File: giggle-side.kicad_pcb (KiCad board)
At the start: 2 copper layers, 97.5 x 97 mm, 41 parts, among them J2 CONN_05X2SHD

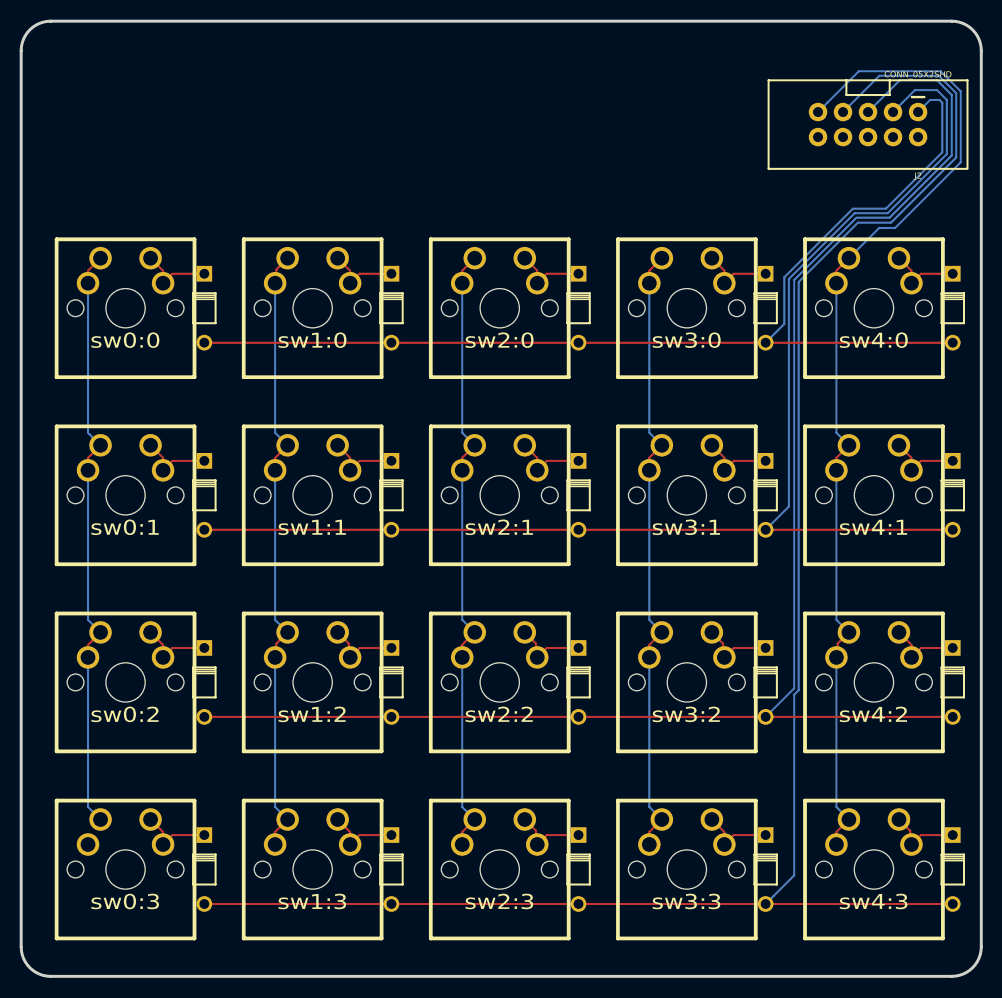
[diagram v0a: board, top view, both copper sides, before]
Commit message: placed the switches and stuff in the main, i guess.
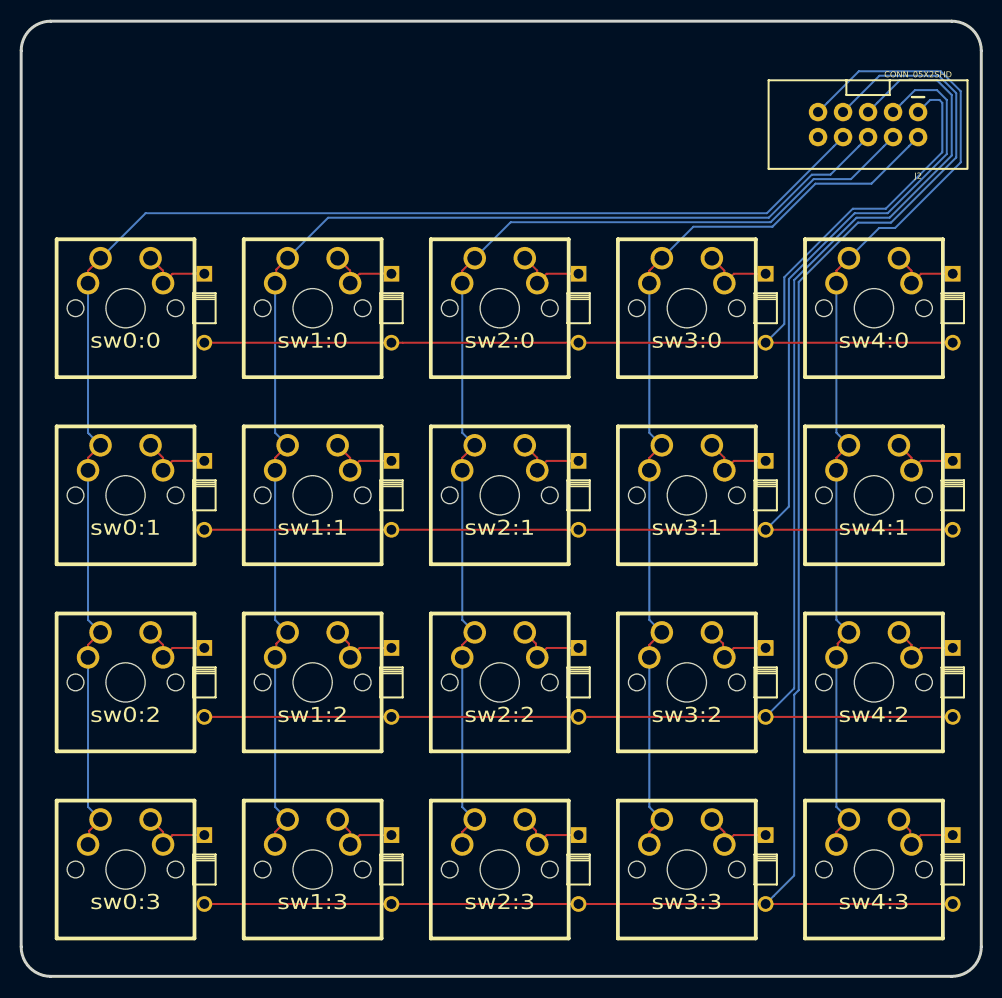
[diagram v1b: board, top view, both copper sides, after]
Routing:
- net N-col-0: track 60.2 -> 143.7 mm
- net N-col-1: track 63.2 -> 127.3 mm
- net N-col-2: track 63.2 -> 110.8 mm
- net N-col-3: track 63.2 -> 94.3 mm
- net N-col-8: track 0.00 -> 7.65 mm
- net N-col-7: track 0.00 -> 7.65 mm
- net N-col-6: track 0.00 -> 7.65 mm
- net N-col-5: track 0.00 -> 7.65 mm
- net N-col-11: track 0.00 -> 7.65 mm
- net N-diode-19: track 7.65 -> 0.00 mm
- net N-diode-14: track 7.65 -> 0.00 mm
- net N-diode-11: track 7.65 -> 0.00 mm
- net N-col-9: track 0.00 -> 7.65 mm
- net N-col-12: track 0.00 -> 7.65 mm
- net N-col-10: track 0.00 -> 7.65 mm
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
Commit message: finished main side.
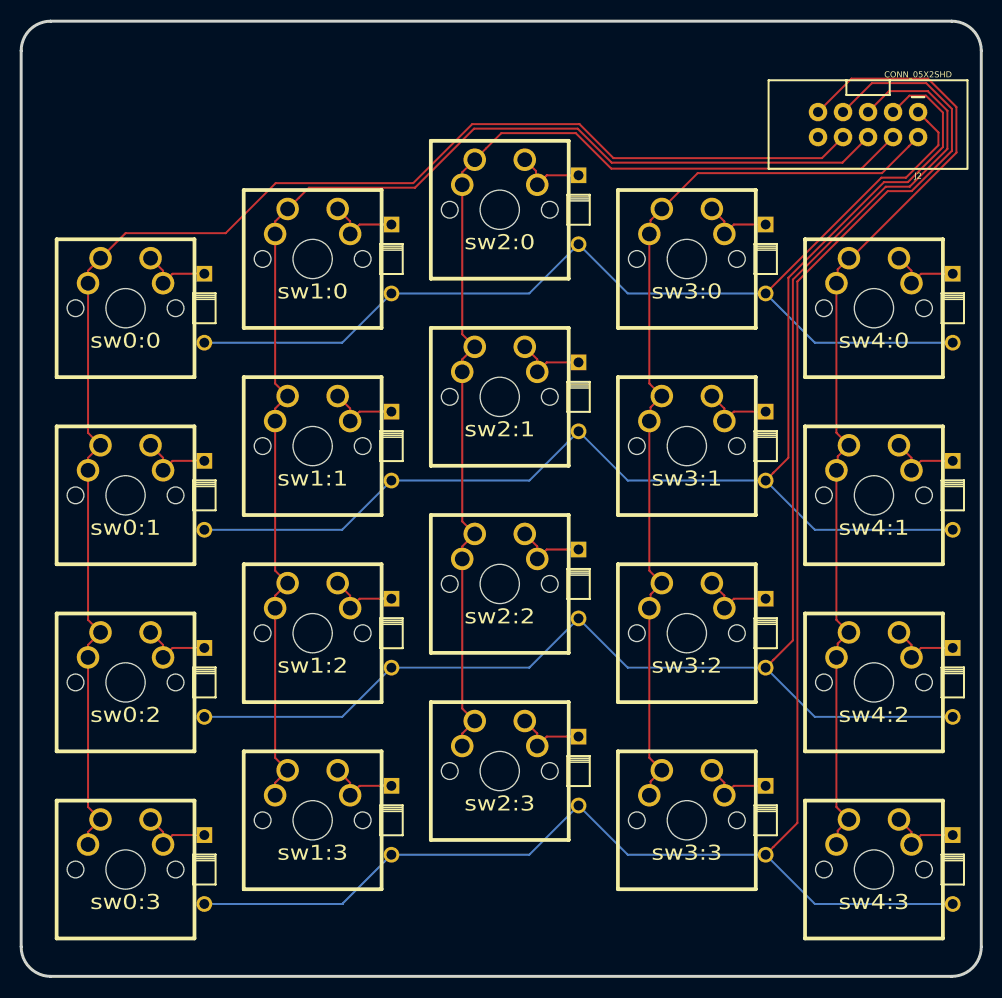
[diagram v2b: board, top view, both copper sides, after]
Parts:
- moved d2:0 10.0 mm to (84.1, 47.1)
- moved d2:1 10.0 mm to (84.1, 66.2)
- moved d2:2 10.0 mm to (84.1, 85.2)
- moved d2:3 10.0 mm to (84.1, 104.2)
- moved sw2:0 10.0 mm to (76.1, 47.1)
- moved sw2:1 10.0 mm to (76.1, 66.2)
- moved sw2:2 10.0 mm to (76.1, 85.2)
- moved sw2:3 10.0 mm to (76.1, 104.2)
- moved d1:0 5.00 mm to (65.1, 52.1)
- moved d1:1 5.00 mm to (65.1, 71.2)
- moved d1:2 5.00 mm to (65.1, 90.2)
- moved d1:3 5.00 mm to (65.1, 109.2)
- moved d3:0 5.00 mm to (103.1, 52.1)
- moved d3:1 5.00 mm to (103.1, 71.2)
- moved d3:2 5.00 mm to (103.1, 90.2)
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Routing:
- net N-col-4: track 102.9 -> 99.9 mm
- net N-col-0: track 143.7 -> 146.6 mm
- net N-col-3: track 94.3 -> 92.3 mm
- net N-col-2: track 110.8 -> 109.6 mm
- net N-row-1: track 136.0 -> 137.0 mm
- net N-row-3: track 182.1 -> 183.0 mm
- net N-col-1: track 127.3 -> 128.0 mm
- net N-row-0: track 112.8 -> 112.3 mm
